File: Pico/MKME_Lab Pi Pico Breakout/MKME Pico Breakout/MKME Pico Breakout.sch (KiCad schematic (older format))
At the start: 1 part

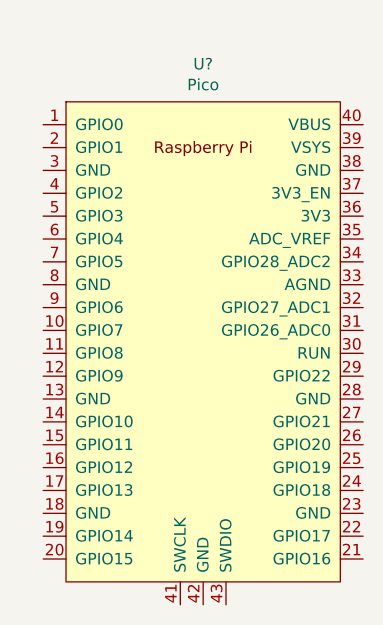
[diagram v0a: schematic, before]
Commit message: pi
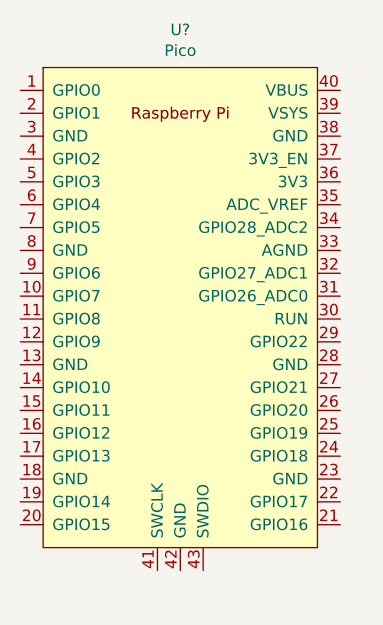
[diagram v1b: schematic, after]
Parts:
- removed U?: Pico, RPi_Pico:RPi_Pico_SMD_TH, symbol MCU_RaspberryPi_and_Boards:Pico
- added U?: Pico, RPi_Pico:RPi_Pico_SMD_TH, symbol MCU_RaspberryPi_and_Boards:Pico
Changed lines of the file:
@@
 $Comp
 L MCU_RaspberryPi_and_Boards:Pico U?
-U 1 1 601B19D6
-P 6100 3600
-F 0 "U?" H 6100 4815 50  0000 C CNN
-F 1 "Pico" H 6100 4724 50  0000 C CNN
-F 2 "RPi_Pico:RPi_Pico_SMD_TH" V 6100 3600 50  0001 C CNN
-F 3 "" H 6100 3600 50  0001 C CNN
-	1    6100 3600
+U 1 1 601B1BD5
+P 6000 3450
+F 0 "U?" H 6000 4665 50  0000 C CNN
+F 1 "Pico" H 6000 4574 50  0000 C CNN
+F 2 "RPi_Pico:RPi_Pico_SMD_TH" V 6000 3450 50  0001 C CNN
+F 3 "" H 6000 3450 50  0001 C CNN
+	1    6000 3450
 	1    0    0    -1
 $EndComp
